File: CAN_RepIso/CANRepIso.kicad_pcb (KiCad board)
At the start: 4 copper layers, 60 x 27 mm, 57 parts, among them U1 SN74LV32ADGVR, U2 SN74LVC2G08DCUR, U3 SN74LVC2G07DBVR, U4 SN74LVC2G04DBVR, U5 SN74LVC2G132DCUR, U6 SN65HVD230, U7 PLACEHOLDER ISOLATOR, U8 SN65HVD230, U9 ADuM120N

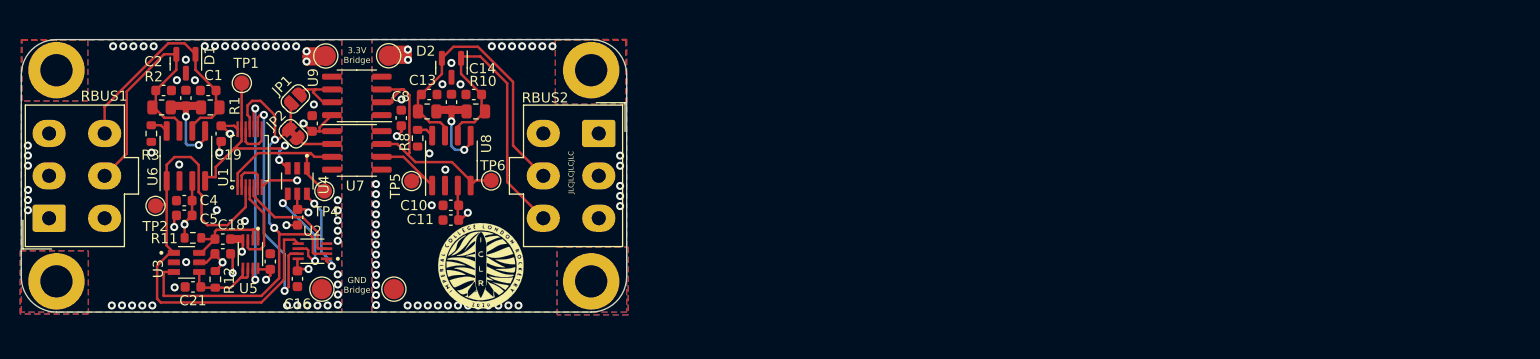
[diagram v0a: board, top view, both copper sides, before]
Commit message: v2 finished pre-review
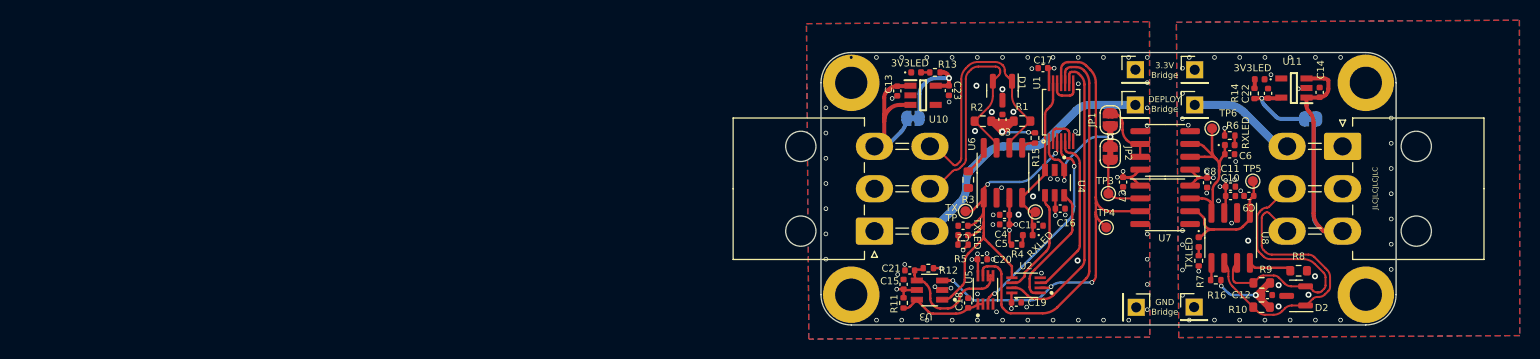
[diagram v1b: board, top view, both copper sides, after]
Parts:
- removed the G*** at (78.3, 104.1)
- added C22: 2.2uF, Capacitor_SMD:C_0402_1005Metric, F.Cu at (156.3, 87.0)
- added C23: 2.2uF, Capacitor_SMD:C_0402_1005Metric, F.Cu at (124.7, 86.8)
- added C6: 1pF, Capacitor_SMD:C_0402_1005Metric, F.Cu at (152.5, 93.1)
- added C9: 1pF, Capacitor_SMD:C_0402_1005Metric, F.Cu at (154.4, 97.2)
- added D3: RX1LED, LED_SMD:LED_0402_1005Metric, F.Cu at (132.5, 101.1)
- added D4: TX1LED, LED_SMD:LED_0402_1005Metric, F.Cu at (126.1, 101.1)
- added D5: RX2LED, LED_SMD:LED_0402_1005Metric, F.Cu at (152.5, 92.2)
- added D6: TX2LED, LED_SMD:LED_0402_1005Metric, F.Cu at (149.4, 101.8)
- added D7: 3V31LED, LED_SMD:LED_0402_1005Metric, F.Cu at (121.4, 85.0)
- added D8: 3V32LED, LED_SMD:LED_0402_1005Metric, F.Cu at (155.5, 85.7)
- added G***: LOGO, LOGO, B.Cu at (122.0, 105.8)
- added JP3: SolderJumper_2_Bridged, Jumper:SolderJumper-2_P1.3mm_Bridged_RoundedPad1.0x1.5mm, B.Cu at (160.5, 89.6)
- added JP4: SolderJumper_2_Bridged, Jumper:SolderJumper-2_P1.3mm_Bridged_RoundedPad1.0x1.5mm, B.Cu at (121.1, 89.5)
- added R13: 470, Resistor_SMD:R_0402_1005Metric, F.Cu at (123.3, 85.0)
- added R14: 470, Resistor_SMD:R_0402_1005Metric, F.Cu at (155.0, 87.1)
- added R15: 0, Resistor_SMD:R_0402_1005Metric, F.Cu at (133.2, 91.5)
- added R16: 0, Resistor_SMD:R_0402_1005Metric, F.Cu at (151.1, 105.5)
- added R4: 1k, Resistor_SMD:R_0402_1005Metric, F.Cu at (131.4, 102.0)
- added R5: 1k, Resistor_SMD:R_0402_1005Metric, F.Cu at (126.1, 102.0)
- added R6: 1k, Resistor_SMD:R_0402_1005Metric, F.Cu at (152.5, 91.2)
- added R7: 1k, Resistor_SMD:R_0402_1005Metric, F.Cu at (149.4, 103.6)
- added TP11: TestPoint, Connector_PinHeader_2.54mm:PinHeader_1x01_P2.54mm_Vertical, F.Cu at (143.2, 88.2)
- added TP12: TestPoint, Connector_PinHeader_2.54mm:PinHeader_1x01_P2.54mm_Vertical, F.Cu at (149.0, 88.2)
- added TP3: TestPoint, TestPoint:TestPoint_Pad_D1.0mm, F.Cu at (140.5, 97.0)
- added U10: AP2205-33W5-7, iclr:SOT95P282X145-5N, F.Cu at (122.1, 87.2)
- added U11: AP2205-33W5-7, iclr:SOT95P282X145-5N, F.Cu at (158.9, 86.5)
- C1: value 220 pF -> 1pF; footprint Capacitor_SMD:C_0603_1608Metric -> Capacitor_SMD:C_0402_1005Metric
- C10, C11, C15, C16, C17, C18, C19, C20, C21, C4, C5, C7, C8: footprint Capacitor_SMD:C_0603_1608Metric -> Capacitor_SMD:C_0402_1005Metric
- C12, C3: value 0.1uF -> 47nF; footprint Capacitor_SMD:C_0603_1608Metric -> Capacitor_SMD:C_0402_1005Metric
- C13: value 220pF -> 1uF; footprint Capacitor_SMD:C_0603_1608Metric -> Capacitor_SMD:C_0402_1005Metric
- C14: value 220 pF -> 1uF; footprint Capacitor_SMD:C_0603_1608Metric -> Capacitor_SMD:C_0402_1005Metric
- C2: value 220pF -> 1pF; footprint Capacitor_SMD:C_0603_1608Metric -> Capacitor_SMD:C_0402_1005Metric
- R1, R10, R2, R9: footprint Resistor_SMD:R_0805_2012Metric -> Resistor_SMD:R_0603_1608Metric
- R11, R12: footprint Resistor_SMD:R_0603_1608Metric -> Resistor_SMD:R_0402_1005Metric
- R3, R8: value 10k -> 0
- RBUS1, RBUS2: footprint Connector_Molex:Molex_Mini-Fit_Jr_5566-06A_2x03_P4.20mm_Vertical -> Connector_Molex:Molex_Mini-Fit_Jr_5569-06A2_2x03_P4.20mm_Horizontal
- TP1, TP2, TP4, TP5, TP6: footprint TestPoint:TestPoint_Pad_D1.5mm -> TestPoint:TestPoint_Pad_D1.0mm
- TP10, TP7, TP8, TP9: footprint TestPoint:TestPoint_Pad_D2.0mm -> Connector_PinHeader_2.54mm:PinHeader_1x01_P2.54mm_Vertical
- moved R8 88.3 mm to (159.3, 104.6), turned to 0 degrees
- moved D2 86.7 mm to (159.1, 107.1), turned to 180 degrees
- moved R9 84.4 mm to (155.7, 105.8)
- moved C14 83.8 mm to (161.4, 87.0), turned to 90 degrees
- moved TP5 83.4 mm to (154.8, 95.8)
- moved C1 83.3 mm to (133.5, 100.2)
- moved C17 83.3 mm to (134.0, 84.5), turned to 180 degrees
- moved C12 83.1 mm to (156.2, 107.0), turned to 0 degrees
- moved RBUS1 81.8 mm to (117.3, 100.7)
- moved G*** 81.6 mm to (146.7, 97.4)
- moved R2 81.4 mm to (128.1, 89.8)
- moved C4 81.3 mm to (130.2, 99.1)
- moved C5 81.3 mm to (130.2, 100.0)
- moved R3 81.1 mm to (126.6, 95.6)
- moved U6 81.0 mm to (130.0, 94.9)
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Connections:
- net Net-(TP5-Pad1) renamed /TX2_PRE_ISO
- net Net-(TP6-Pad1) renamed /RX2_PRE_ISO
- C1 pad 1: GND -> /RX1
- C1 pad 2: /CAN_LOW_IN -> GND
- C13 pad 1: GND1 -> /RBUS_uC_V1
- C13 pad 2: /CAN_HIGH_OUT -> GND
- C14 pad 1: GND1 -> /RBUS_uC_V2
- C14 pad 2: /CAN_LOW_OUT -> GND1
- C2 pad 1: GND -> /TX1
- C2 pad 2: /CAN_HIGH_IN -> GND
- D1 pad 1: /CAN_LOW_IN -> /CAN_IN_-
- D1 pad 2: /CAN_HIGH_IN -> /CAN_IN_+
- D2 pad 1: /CAN_LOW_OUT -> /CAN_OUT_-
- D2 pad 2: /CAN_HIGH_OUT -> /CAN_OUT_+
- JP1 pad 1: /RX2 -> /TX2
- JP2 pad 1: /RX2 -> /TX2
- R1 pad 2: /CAN_LOW_IN -> /CAN_IN_-
- R10 pad 2: /CAN_LOW_OUT -> /CAN_OUT_-
- R2 pad 1: /CAN_HIGH_IN -> /CAN_IN_+
- R9 pad 1: /CAN_HIGH_OUT -> /CAN_OUT_+
- RBUS1 pad 3: +3V3 -> /RBUS_uC_V1
- RBUS1 pad 4: unconnected-(RBUS1-Pad4) -> /Deploy1
- RBUS1 pad 5: /CAN_HIGH_IN -> /CAN_IN_+
- RBUS1 pad 6: /CAN_LOW_IN -> /CAN_IN_-
- RBUS2 pad 3: +3.3VA -> /RBUS_uC_V2
- RBUS2 pad 4: unconnected-(RBUS2-Pad4) -> /Deploy2
- RBUS2 pad 5: /CAN_HIGH_OUT -> /CAN_OUT_+
- RBUS2 pad 6: /CAN_LOW_OUT -> /CAN_OUT_-
- TP4 pad 1: /TX2 -> /RX2
- U6 pad 5: /Vref -> Net-(U6-Vref)
- U6 pad 6: /CAN_LOW_IN -> /CAN_IN_-
- U6 pad 7: /CAN_HIGH_IN -> /CAN_IN_+
- U7 pad 3: /TX2 -> /RX2
- U8 pad 5: /Vref2 -> Net-(U8-Vref)
- U8 pad 6: /CAN_LOW_OUT -> /CAN_OUT_-
- U8 pad 7: /CAN_HIGH_OUT -> /CAN_OUT_+
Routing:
- net /RBUS_uC_V2: track 0.00 -> 34.8 mm
- net /CAN_LOW_OUT: track 30.6 -> 0.00 mm
- net /CAN_OUT_-: track 0.00 -> 29.8 mm
- net /CAN_HIGH_OUT: track 29.0 -> 0.00 mm
- net /CAN_OUT_+: track 0.00 -> 28.3 mm
- net /CAN_IN_-: track 0.00 -> 27.2 mm
- net /CAN_IN_+: track 0.00 -> 26.6 mm
- net /Deploy1: track 0.00 -> 26.3 mm
- net /CAN_HIGH_IN: track 24.6 -> 0.00 mm
- net /CAN_LOW_IN: track 23.8 -> 0.00 mm
- net Net-(U1-3B): track 20.4 -> 40.3 mm, vias 2 -> 0
- net /RBUS_uC_V1: track 0.00 -> 16.7 mm
- net /TX1: track 50.9 -> 35.7 mm, vias 0 -> 2
- net Net-(U1-2A): track 8.98 -> 20.4 mm, vias 0 -> 2
- net /Deploy2: track 0.00 -> 10.7 mm
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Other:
- board size 60 x 27 mm -> 57 x 27 mm
- board text added: "DEPLOY Bridge"
- board text added: "Designed By Andrei Paduraru Electronics and Payload 2023"
- board text added: "REPEATER 2.0"
- board text added: "THE COULDN'T"
- board text removed: "CAN BUS REPEATER"
- board text removed: "Designed By Andrei Paduraru Electronics and Payload 2022"
- board text removed: "Isolator?"
- board text removed: "No"
- board text removed: "Yes"
